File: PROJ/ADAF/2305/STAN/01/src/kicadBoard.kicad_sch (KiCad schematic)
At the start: 23 parts

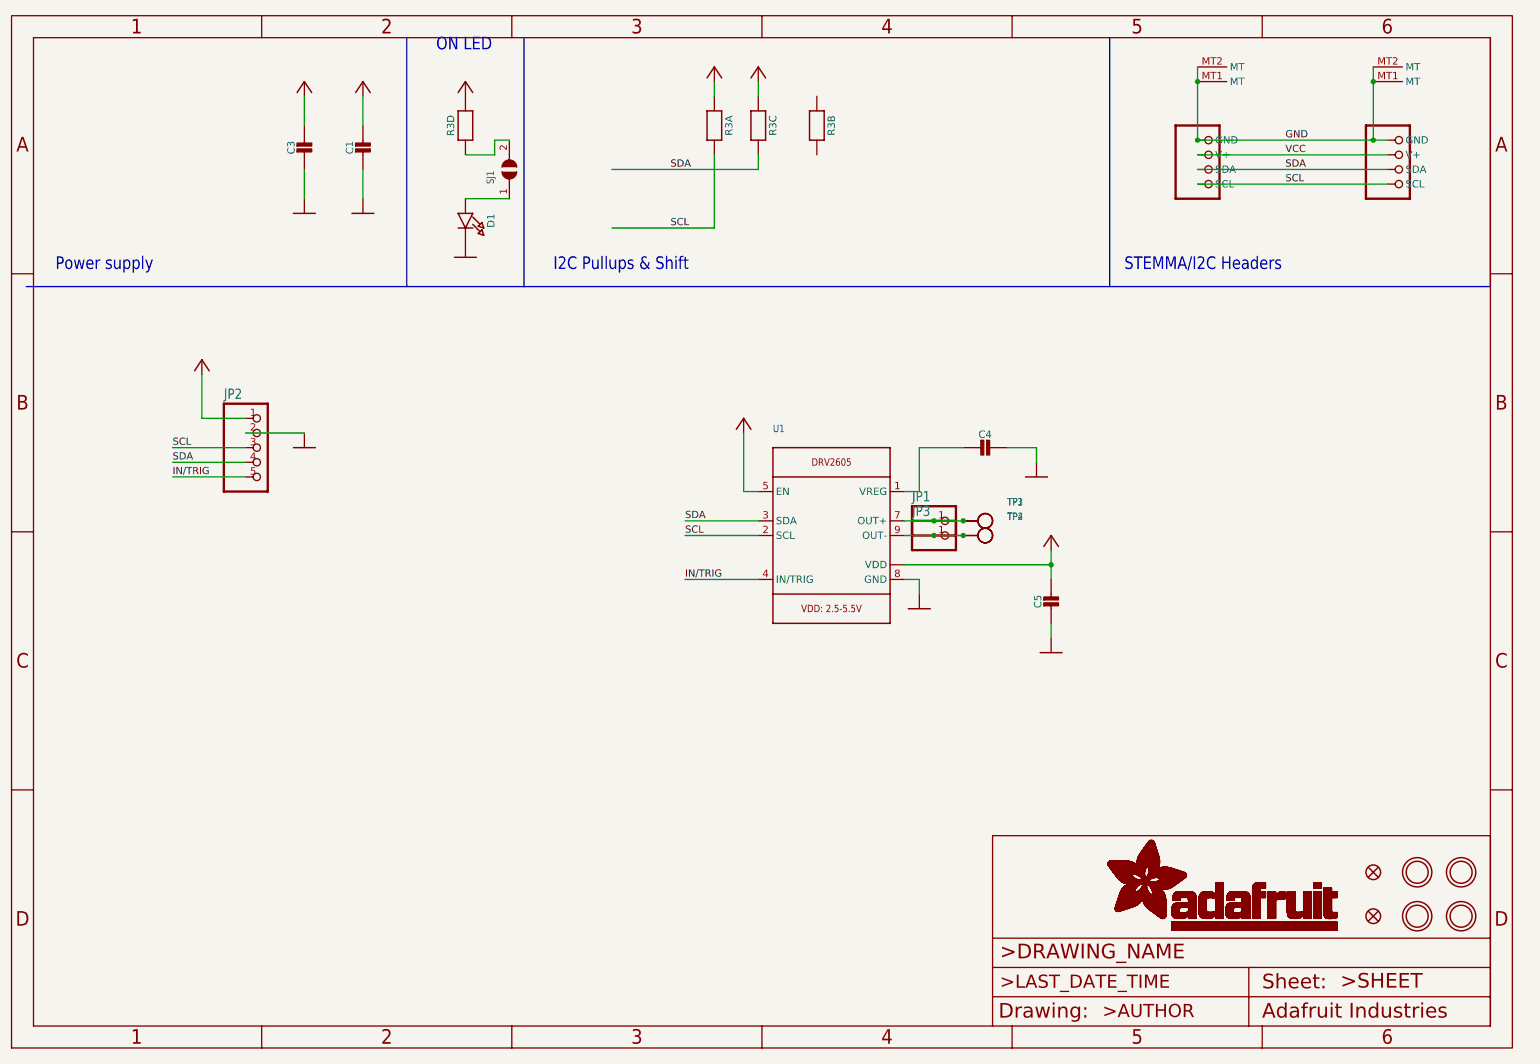
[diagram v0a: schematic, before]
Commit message: Quickly Adding Everything
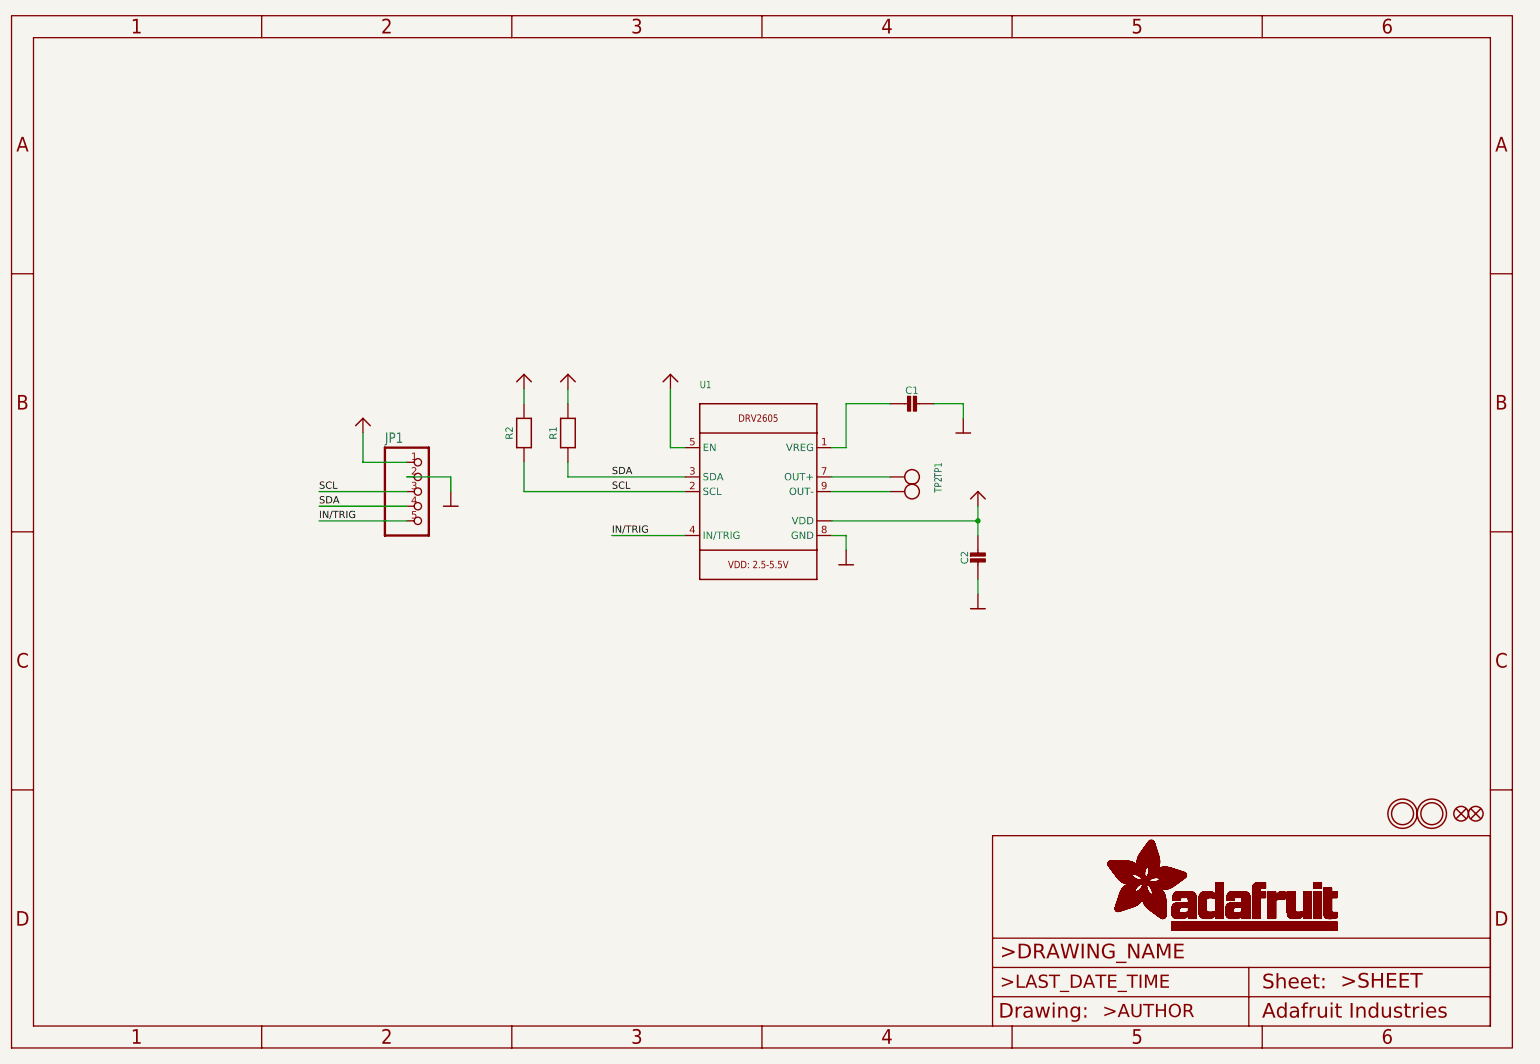
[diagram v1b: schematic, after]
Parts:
- removed C1, C4, C5: (no value), symbol eagleSchem-eagle-import:CAP_CERAMIC0603_NO
- removed C3: (no value), symbol eagleSchem-eagle-import:CAP_CERAMIC0805-NOOUTLINE
- removed CONN3, CONN4: (no value), symbol eagleSchem-eagle-import:STEMMA_I2C_QT
- removed D1: (no value), symbol eagleSchem-eagle-import:LED0603_NOOUTLINE
- removed FID3, FID4: (no value), symbol eagleSchem-eagle-import:FIDUCIAL_1MM
- removed JP1, JP3: (no value), symbol eagleSchem-eagle-import:HEADER-1X1
- removed JP2: (no value), symbol eagleSchem-eagle-import:HEADER-1X576MIL
- removed R3: (no value), symbol eagleSchem-eagle-import:RESISTOR_4PACK
- removed SJ1: (no value), symbol eagleSchem-eagle-import:SOLDERJUMPERCLOSED
- removed TP1, TP2, TP3, TP4: (no value), symbol eagleSchem-eagle-import:TESTPOINTPAD2MM
- removed U$1, U$17, U$19, U$21: (no value), symbol eagleSchem-eagle-import:MOUNTINGHOLE2.5
- removed U1: (no value), symbol eagleSchem-eagle-import:DRV2605_SOP
- added C1, C2: (no value), symbol schematicEagle-eagle-import:CAP_CERAMIC0805-NOOUTLINE
- added FID1, FID2: (no value), symbol schematicEagle-eagle-import:FIDUCIAL{dblquote}{dblquote}
- added JP1: (no value), symbol schematicEagle-eagle-import:HEADER-1X576MIL_FULL
- added R1, R2: (no value), symbol schematicEagle-eagle-import:RESISTOR0805_NOOUTLINE
- added TP1, TP2: (no value), symbol schematicEagle-eagle-import:TESTPOINTPAD2MM
- added U$2, U$3: (no value), symbol schematicEagle-eagle-import:MOUNTINGHOLE2.5
- added U1: (no value), symbol schematicEagle-eagle-import:DRV2605_SOP
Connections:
- net GND: now also C1.1, C2.2, JP1.2, U1.8 (GND)
- net IN/TRIG: now also JP1.5, U1.4 (IN/TRIG)
- net SCL: now also JP1.3, R2.1, U1.2 (SCL)
- net SDA: now also JP1.4, R1.1, U1.3 (SDA)
- new net: TP2.P$1, U1.9 (OUT-)
- new net: TP1.P$1, U1.7 (OUT+)
- new net: C1.2, U1.1 (VREG)
- new net VIN: C2.1, JP1.1, R1.2, R2.2, U1.10 (VDD), U1.5 (EN), U1.6 (VDD)
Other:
- note removed: "I2C Pullups & Shift"
- note removed: "ON LED"
- note removed: "Power supply"
- note removed: "STEMMA/I2C Headers"

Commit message: Quickly Adding Everything
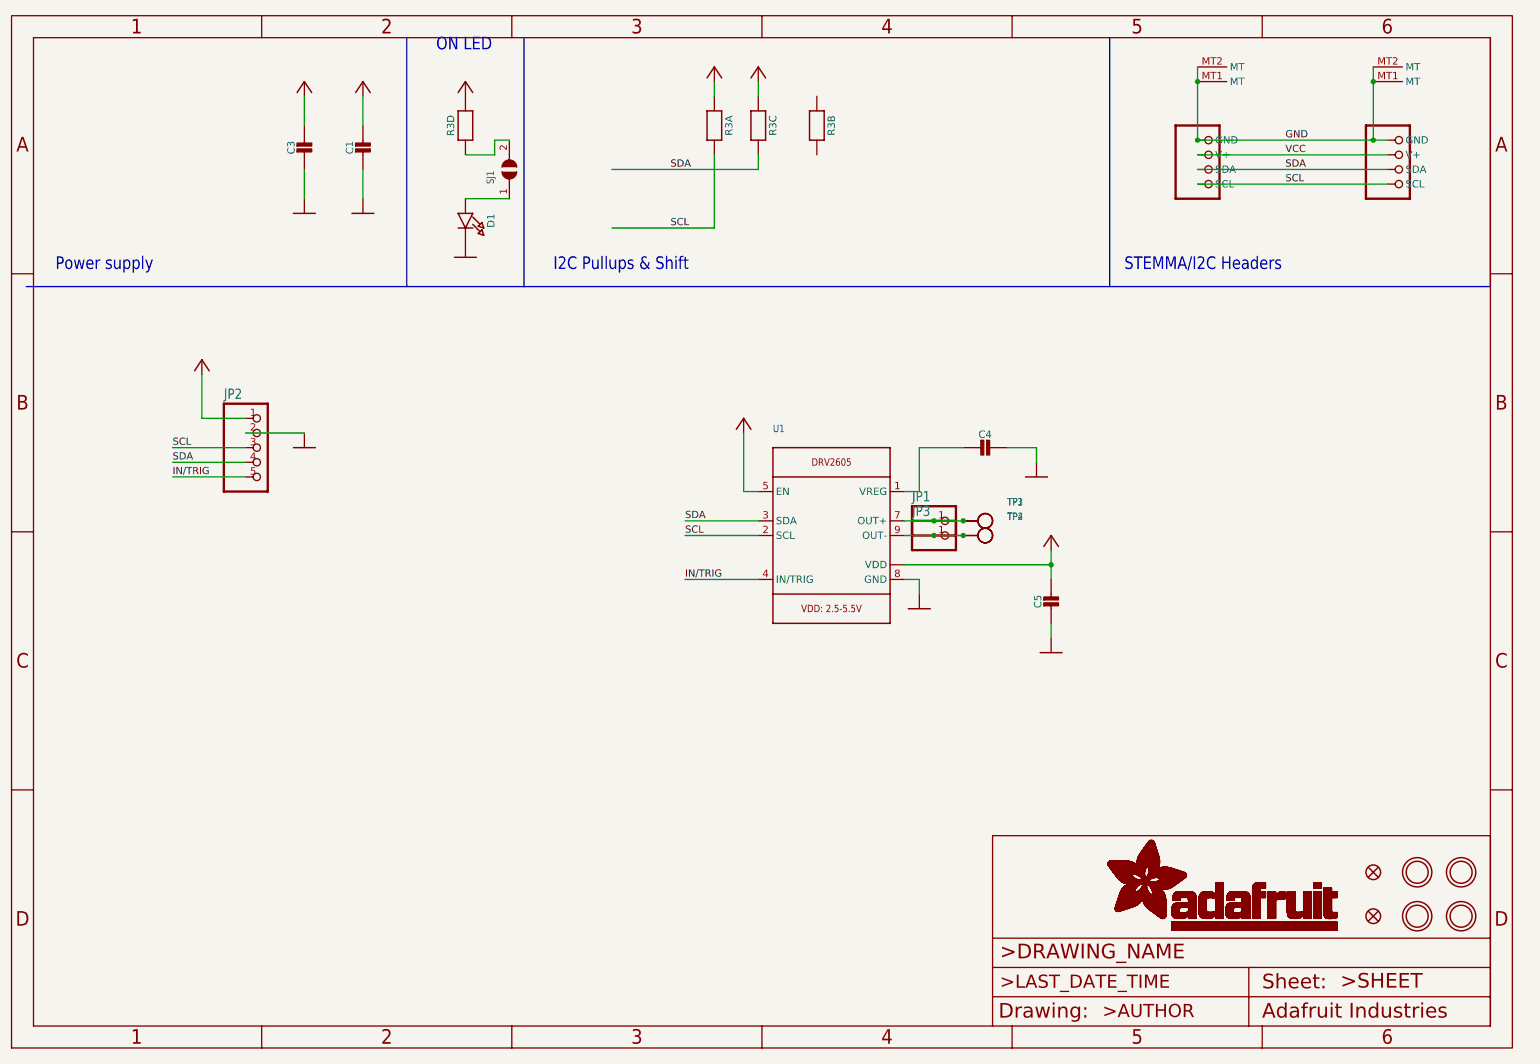
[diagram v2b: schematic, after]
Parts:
- removed C1, C2: (no value), symbol schematicEagle-eagle-import:CAP_CERAMIC0805-NOOUTLINE
- removed FID1, FID2: (no value), symbol schematicEagle-eagle-import:FIDUCIAL{dblquote}{dblquote}
- removed JP1: (no value), symbol schematicEagle-eagle-import:HEADER-1X576MIL_FULL
- removed R1, R2: (no value), symbol schematicEagle-eagle-import:RESISTOR0805_NOOUTLINE
- removed TP1, TP2: (no value), symbol schematicEagle-eagle-import:TESTPOINTPAD2MM
- removed U$2, U$3: (no value), symbol schematicEagle-eagle-import:MOUNTINGHOLE2.5
- removed U1: (no value), symbol schematicEagle-eagle-import:DRV2605_SOP
- added C1, C4, C5: (no value), symbol eagleSchem-eagle-import:CAP_CERAMIC0603_NO
- added C3: (no value), symbol eagleSchem-eagle-import:CAP_CERAMIC0805-NOOUTLINE
- added CONN3, CONN4: (no value), symbol eagleSchem-eagle-import:STEMMA_I2C_QT
- added D1: (no value), symbol eagleSchem-eagle-import:LED0603_NOOUTLINE
- added FID3, FID4: (no value), symbol eagleSchem-eagle-import:FIDUCIAL_1MM
- added JP1, JP3: (no value), symbol eagleSchem-eagle-import:HEADER-1X1
- added JP2: (no value), symbol eagleSchem-eagle-import:HEADER-1X576MIL
- added R3: (no value), symbol eagleSchem-eagle-import:RESISTOR_4PACK
- added SJ1: (no value), symbol eagleSchem-eagle-import:SOLDERJUMPERCLOSED
- added TP1, TP2, TP3, TP4: (no value), symbol eagleSchem-eagle-import:TESTPOINTPAD2MM
- added U$1, U$17, U$19, U$21: (no value), symbol eagleSchem-eagle-import:MOUNTINGHOLE2.5
- added U1: (no value), symbol eagleSchem-eagle-import:DRV2605_SOP
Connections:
- net GND: now also C1.2, C3.2, C4.1, C5.2, CONN3.1 (GND), CONN3.MT1 (MT), CONN3.MT2 (MT), CONN4.1 (GND), CONN4.MT1 (MT), CONN4.MT2 (MT), D1.C, JP2.2, U1.8 (GND)
- net IN/TRIG: now also JP2.5, U1.4 (IN/TRIG)
- net SCL: now also CONN3.4 (SCL), CONN4.4 (SCL), JP2.3, R3.8 (2), U1.2 (SCL)
- net SDA: now also CONN3.3 (SDA), CONN4.3 (SDA), JP2.4, R3.6 (2), U1.3 (SDA)
- new net: C4.2, U1.1 (VREG)
- new net: JP1.1, TP1.P$1, TP3.P$1, U1.7 (OUT+)
- new net: JP3.1, TP2.P$1, TP4.P$1, U1.9 (OUT-)
- new net: D1.A, SJ1.1
- new net: R3.4 (1), SJ1.2
- new net VCC: C1.1, C3.1, C5.1, CONN3.2 (V+), CONN4.2 (V+), JP2.1, R3.1, R3.3 (1), R3.5 (2), U1.10 (VDD), U1.5 (EN), U1.6 (VDD)
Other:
- note added: "I2C Pullups & Shift"
- note added: "ON LED"
- note added: "Power supply"
- note added: "STEMMA/I2C Headers"
